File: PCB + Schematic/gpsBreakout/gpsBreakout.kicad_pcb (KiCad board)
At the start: 2 copper layers, 18.7 x 27.1 mm, 18 parts, among them J1 Header, U1 ATGM336H, U2 AT24CS32-STUM, U3 AT2659

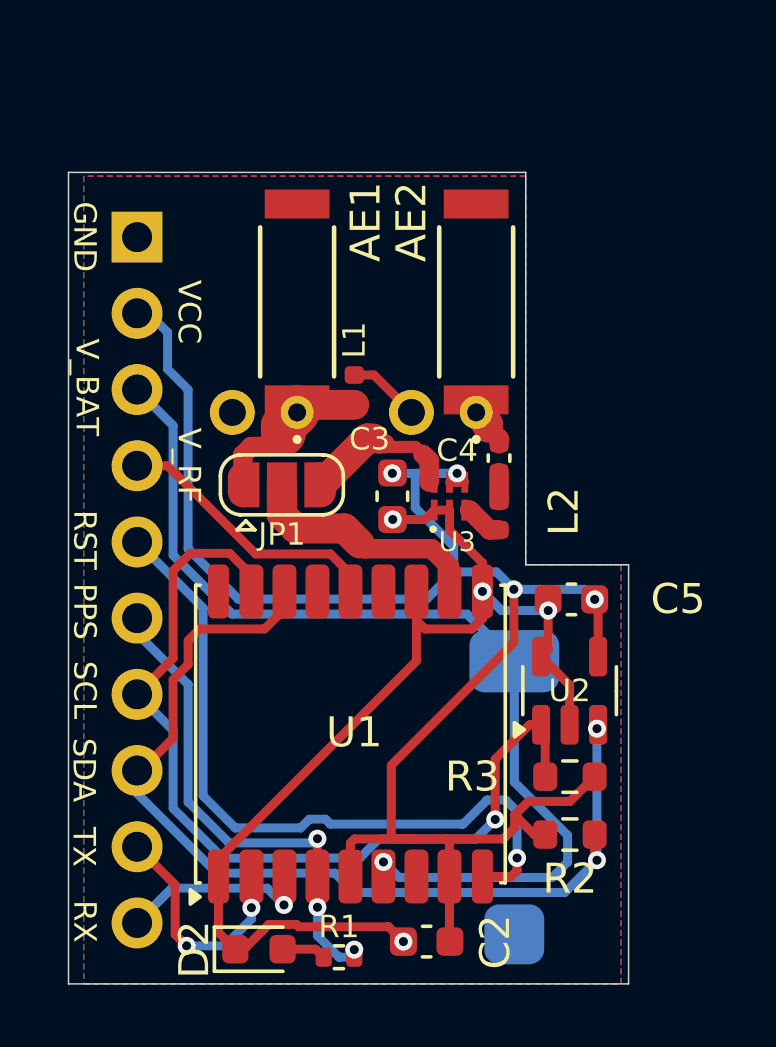
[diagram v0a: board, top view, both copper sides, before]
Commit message: Actually finished board, did GPS work
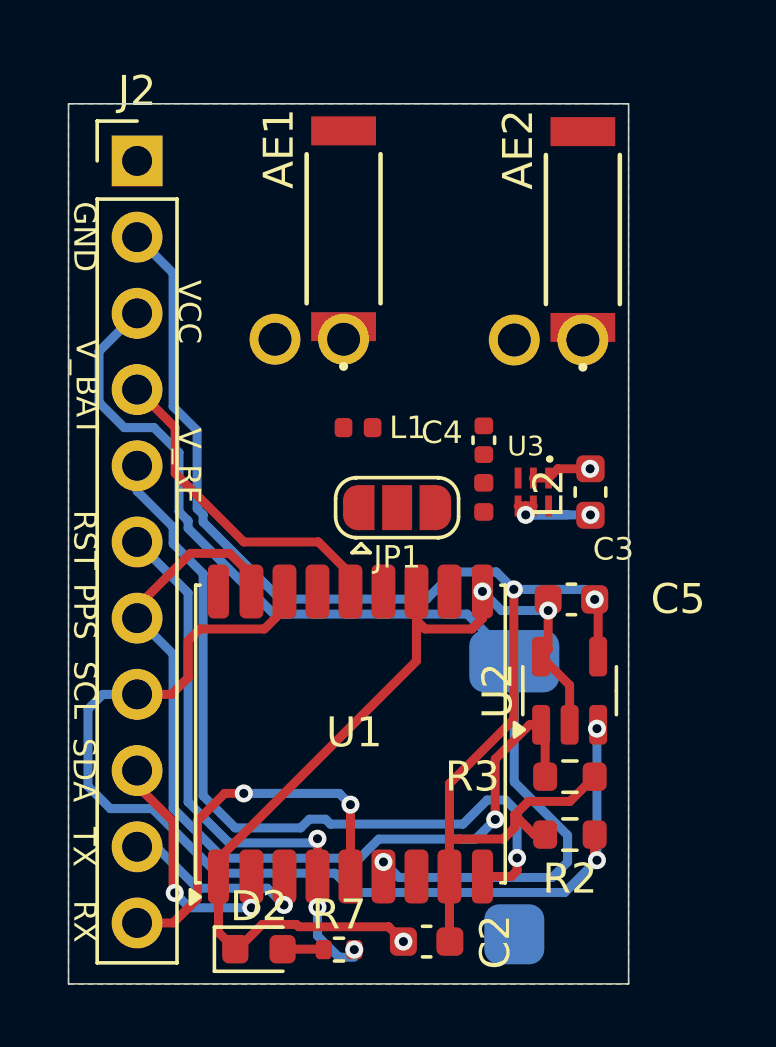
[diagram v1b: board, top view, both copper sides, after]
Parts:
- removed J1: Header, footprints:PinHeader_1x10_P2.54mm_Vertical
- removed R1: 1 K, footprints:R_0402_1005Metric
- added J2: Header, Connector_PinHeader_2.54mm:PinHeader_1x11_P2.54mm_Vertical, F.Cu at (142.0, 77.0)
- added R7: 1 K, Resistor_SMD:R_0402_1005Metric, F.Cu at (148.7, 103.3)
- D2: value RED -> YELLOW; footprint footprints:LED_0603_1608Metric -> LED_SMD:LED_0603_1608Metric
- U2: value AT24CS32-STUM -> BL24C32F-RRRC; footprint footprints:SOT-23-5 -> Package_TO_SOT_SMD:SOT-23-5
- moved C3 6.61 mm to (157.1, 88.0), turned to 90 degrees
- moved AE2 4.30 mm to (156.8, 79.2)
- moved JP1 3.91 mm to (150.7, 88.5)
- moved AE1 2.89 mm to (148.9, 79.2)
- moved U3 2.80 mm to (155.2, 88.0), turned to -90 degrees
- moved L1 1.28 mm to (149.4, 85.9), turned to 0 degrees
- moved C4 0.78 mm to (153.5, 86.3)
- moved L2 0.78 mm to (153.5, 88.2)
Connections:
- net VBAT renamed V_BAT
- U1 pad 5: +3.3V -> GPS_EN
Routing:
- net GPS_EN: track 0.00 -> 13.0 mm, vias 0 -> 2
- net RF: track 8.85 -> 0.00 mm
- net +3.3V: track 59.9 -> 51.5 mm
- net PASSIVE: track 6.13 -> 0.00 mm
- net ACTIVE: track 5.60 -> 0.00 mm
- net GND: track 39.1 -> 33.5 mm
- net V_BAT: track 33.3 -> 37.1 mm
- net SDA: track 32.8 -> 36.3 mm
- net RESET: track 24.2 -> 26.7 mm
- net PPS: track 16.5 -> 19.1 mm
- net Net-(AE2-FEED): track 2.06 -> 0.00 mm
- net VCC_RF: track 9.19 -> 11.1 mm
- net Net-(U3-RF_IN): track 1.25 -> 0.00 mm
- net Net-(C4-Pad2): track 0.94 -> 0.00 mm
- net SCL: track 30.4 -> 31.0 mm
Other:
- board size 18.7 x 27.1 mm -> 18.7 x 29.3 mm

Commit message: Work on GPS
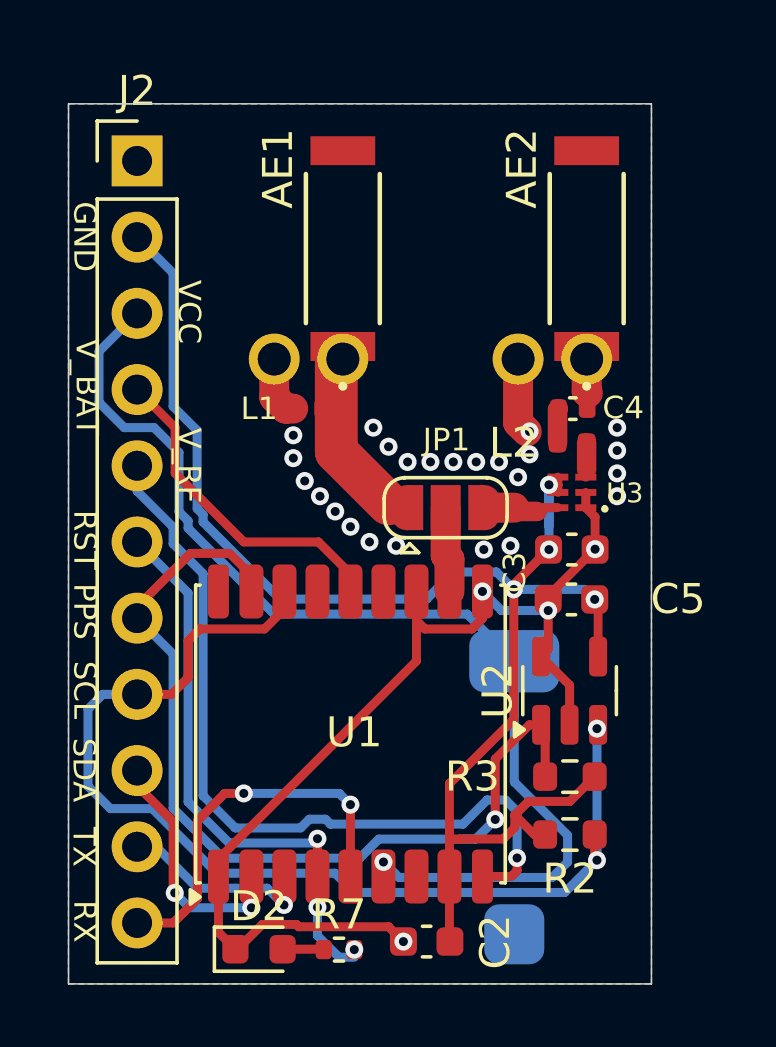
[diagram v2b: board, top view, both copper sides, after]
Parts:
- moved L2 3.46 mm to (156.5, 86.4), turned to 0 degrees
- moved C4 3.15 mm to (156.5, 85.2), turned to 180 degrees
- moved C3 2.02 mm to (156.5, 89.9), turned to 0 degrees
- moved L1 1.77 mm to (147.7, 85.2), turned to 180 degrees
- moved JP1 1.62 mm to (152.3, 88.5)
- moved U3 1.28 mm to (156.5, 88.0), turned to 180 degrees
- moved AE1 0.66 mm to (148.8, 79.9)
- moved AE2 0.65 mm to (157.0, 79.9)
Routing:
- net GND: track 33.5 -> 40.5 mm, vias 4 -> 28
- net PASSIVE: track 0.00 -> 6.29 mm
- net RF: track 0.00 -> 2.85 mm
- net ACTIVE: track 0.00 -> 2.54 mm
- net +3.3V: track 51.5 -> 53.3 mm
- net Net-(U3-RF_IN): track 0.00 -> 1.16 mm
- net Net-(C4-Pad2): track 0.00 -> 1.15 mm
- net Net-(AE2-FEED): track 0.00 -> 1.14 mm
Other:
- board size 18.7 x 29.3 mm -> 19.4 x 29.3 mm
